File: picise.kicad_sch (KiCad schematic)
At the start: 38 parts, among them J1 ANT_SMA, J2 SSQ-120-03_GPIO, J3 TSM-103-01-L-SV, U1 MAX-M10S, U2 PCA9557PW, U3 CAT24C256

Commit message: rev2 draft routed
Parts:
- removed J3: TSM-103-01-L-SV, Connector_PinHeader_2.54mm:PinHeader_1x02_P2.54mm_Vertical_SMD_Pin1Right, symbol Connector_Generic:Conn_01x02
- removed JP1: TSM-103-01-L-SV, Connector_PinHeader_2.54mm:PinHeader_1x02_P2.54mm_Vertical_SMD_Pin1Right, symbol Jumper:Jumper_2_Bridged
- added C10, C11: 10uF, Capacitor_SMD:C_0603_1608Metric, symbol Device:C_Small
- added C12: 1uF, Capacitor_SMD:C_0603_1608Metric, symbol Device:C_Small
- added C13: 0.1uF, Capacitor_SMD:C_0603_1608Metric, symbol Device:C_Small
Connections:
- net +3V3: now also C10.1, C11.1, C12.1, C13.1
- net GND: now also C10.2, C11.2, C12.2, C13.2
- net at C1.1, C15.2, J1.1: now also L1.1
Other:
- note removed: "Fan header"
- moved on the sheet: BT1, C14, D25, D42, D69, DS1, JP3, R10, R11, R12, R8, R9

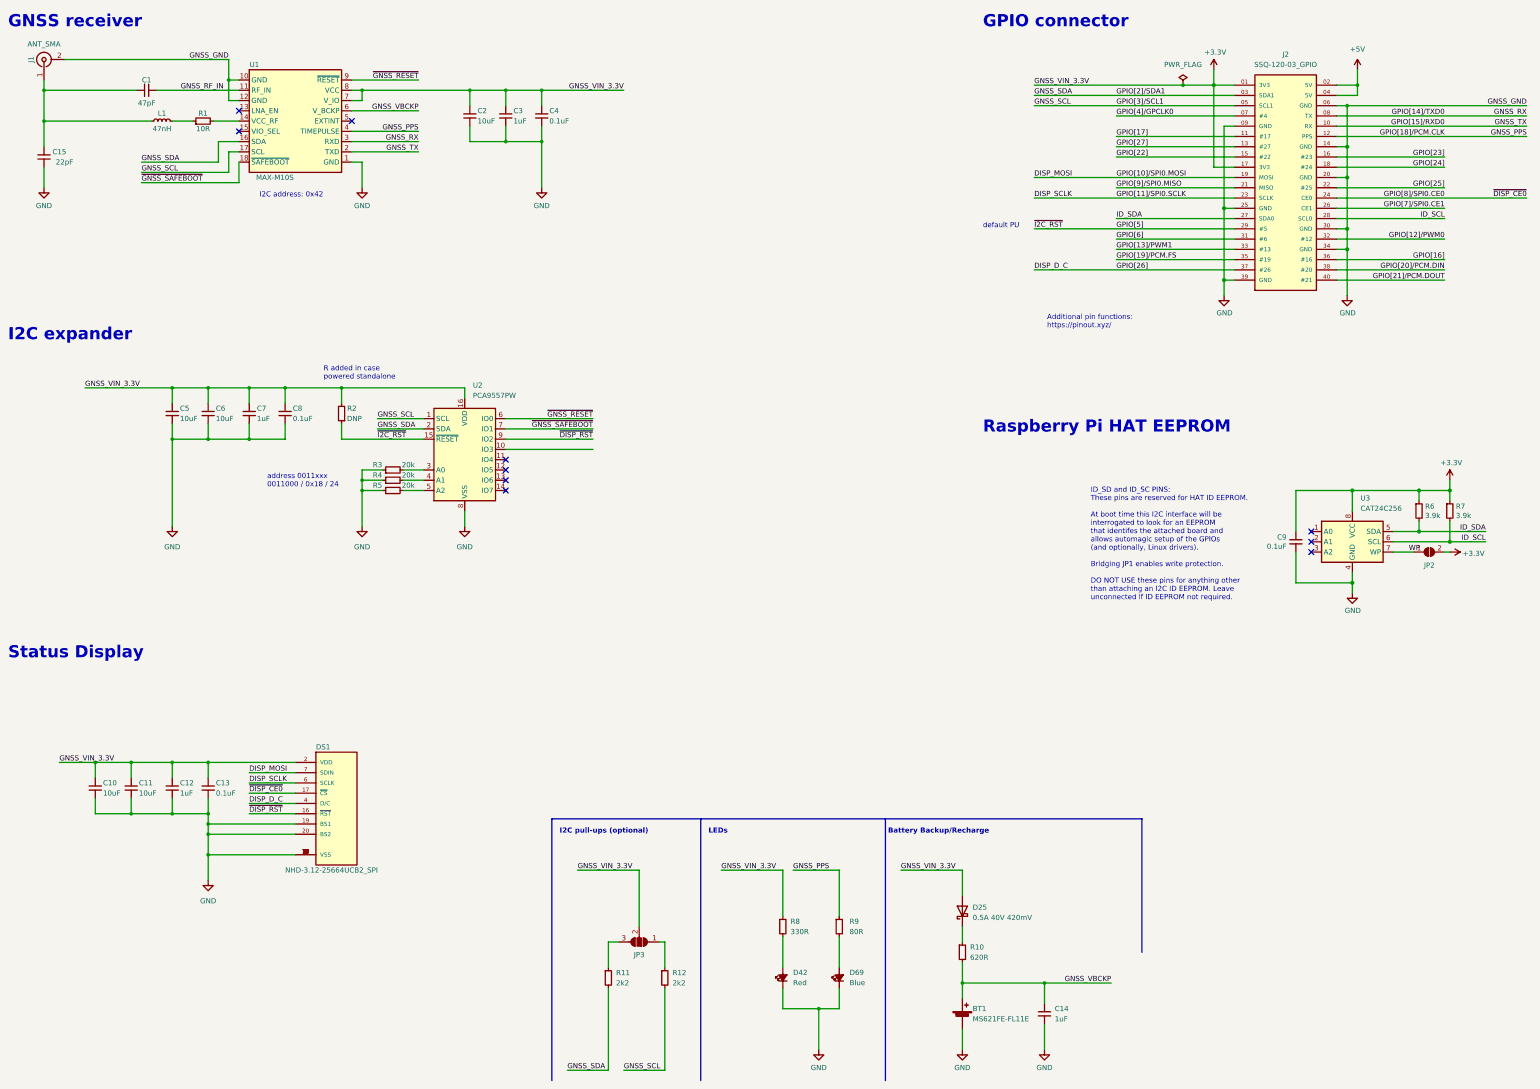
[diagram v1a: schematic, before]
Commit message: tweaks
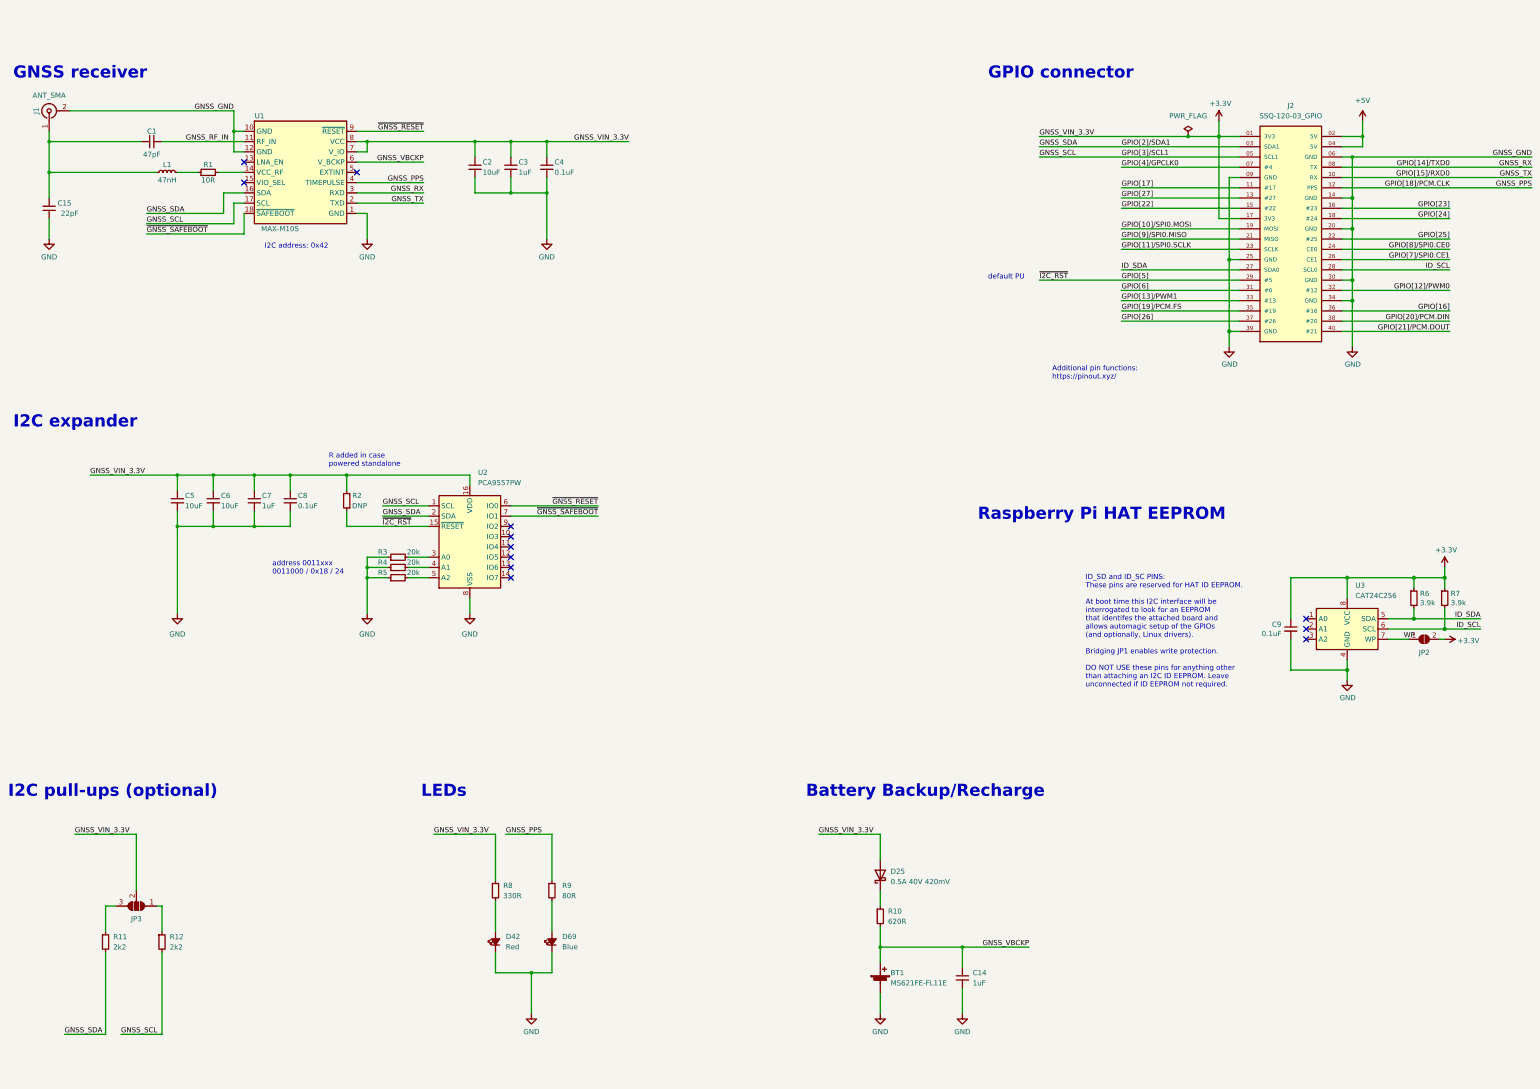
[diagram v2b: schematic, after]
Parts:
- removed C10, C11: 10uF, Capacitor_SMD:C_0603_1608Metric, symbol Device:C_Small
- removed C12: 1uF, Capacitor_SMD:C_0603_1608Metric, symbol Device:C_Small
- removed C13: 0.1uF, Capacitor_SMD:C_0603_1608Metric, symbol Device:C_Small
- removed DS1: NHD-3.12-25664UCB2_SPI, Display_OLED_Newhaven:OLED_NHD-3.12-25664UCx2, symbol Display_OLED_Newhaven:NHD-3.12-25664UCB2_SPI
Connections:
- net DISP_D_C renamed GPIO[26]
- net DISP_MOSI renamed GPIO[10]/SPI0.MOSI
- net DISP_SCLK renamed GPIO[11]/SPI0.SCLK
- net ~{DISP_RST}: no longer names the net of U2.9 (IO2)
- no-connect marks 10 -> 12
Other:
- note removed: "Status Display"
- moved on the sheet: BT1, C1, C14, C15, C2, C3, C4, C5, C6, C7, C8, C9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
